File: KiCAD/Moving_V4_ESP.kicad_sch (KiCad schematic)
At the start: 88 parts, among them J1 Vin_1, J10 Conn_01x03_Pin, J11 Conn_01x03_Pin, J12 Conn_01x03_Pin, J13 Conn_01x03_Pin, J3 Power_SW, J4 USB_B_Micro, J5 MOTOR_R, J6 Motor_L, J7 Conn_01x04_Pin, J8 Conn_01x04_Pin, J9 Vin_XT, Q1 U4_ALT2, Q2 U4_ALT2, Q3 U4_ALT2, SW1 SW_Reset, U1 CH340X, U10 TXB0104RUT, U2 UZ1085L-33-TN3-R, U3 ESP32-WROOM-32, U4 ITR8307-S17-TR8, U5 ITR8307-S17-TR8, U6 ITR8307-S17-TR8, U7 CP3119MDTR, U8 CP2119LDTR, U9 SE8650K2B-HF

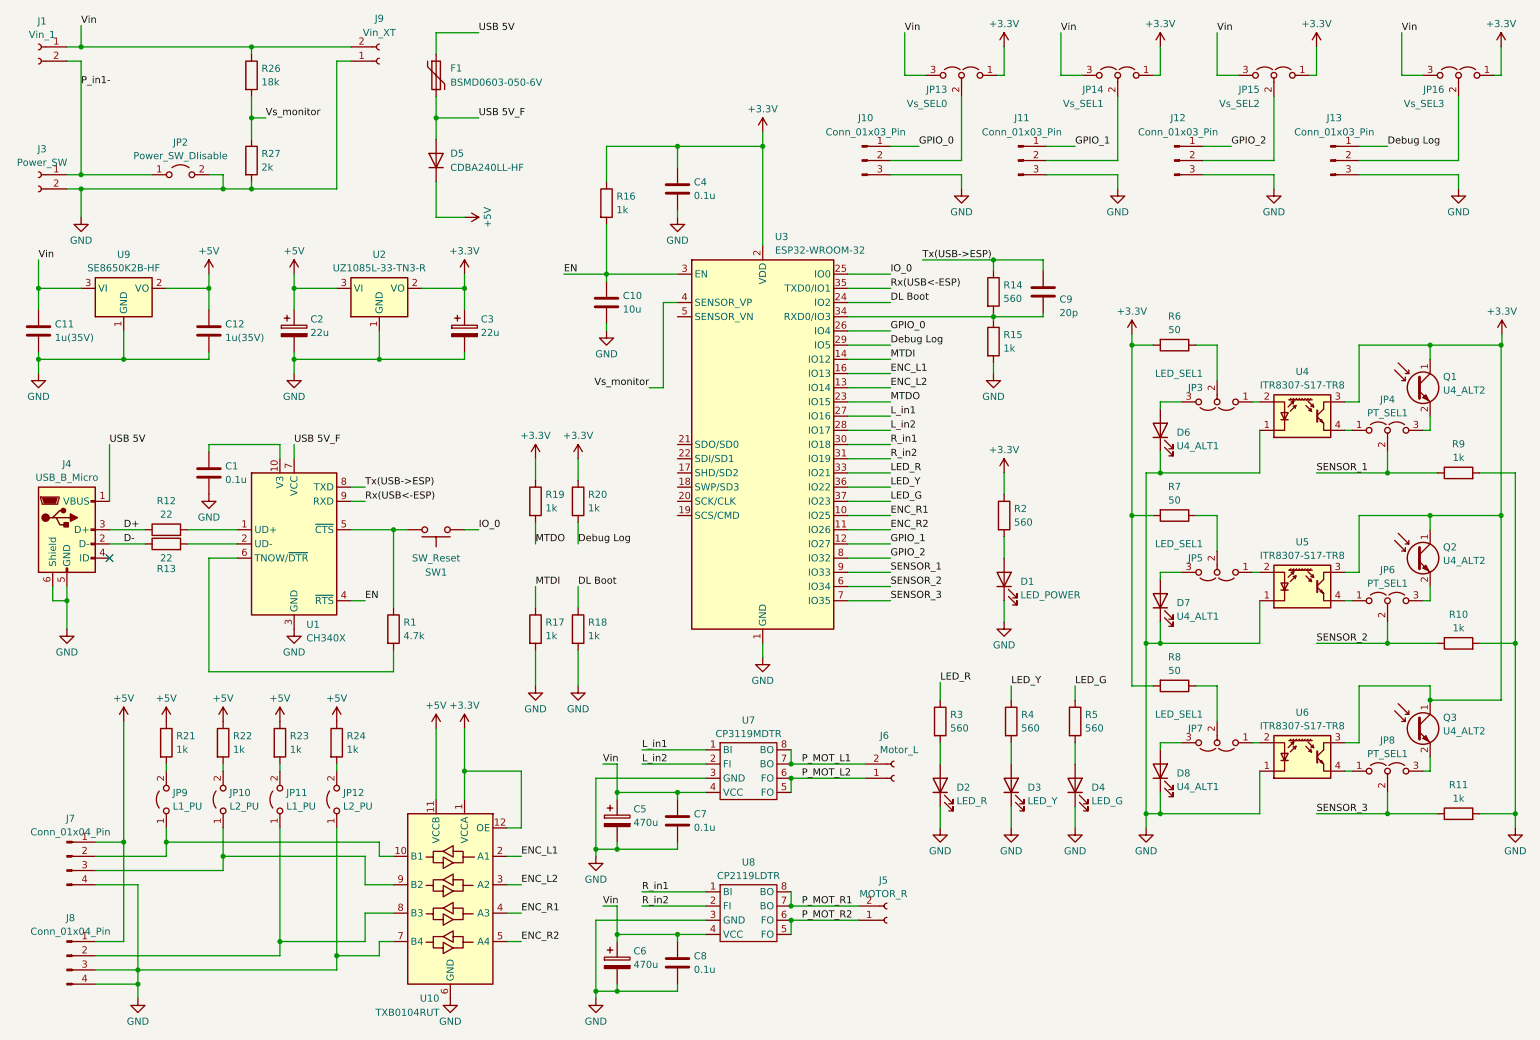
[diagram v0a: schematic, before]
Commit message: アノテーションを再実行
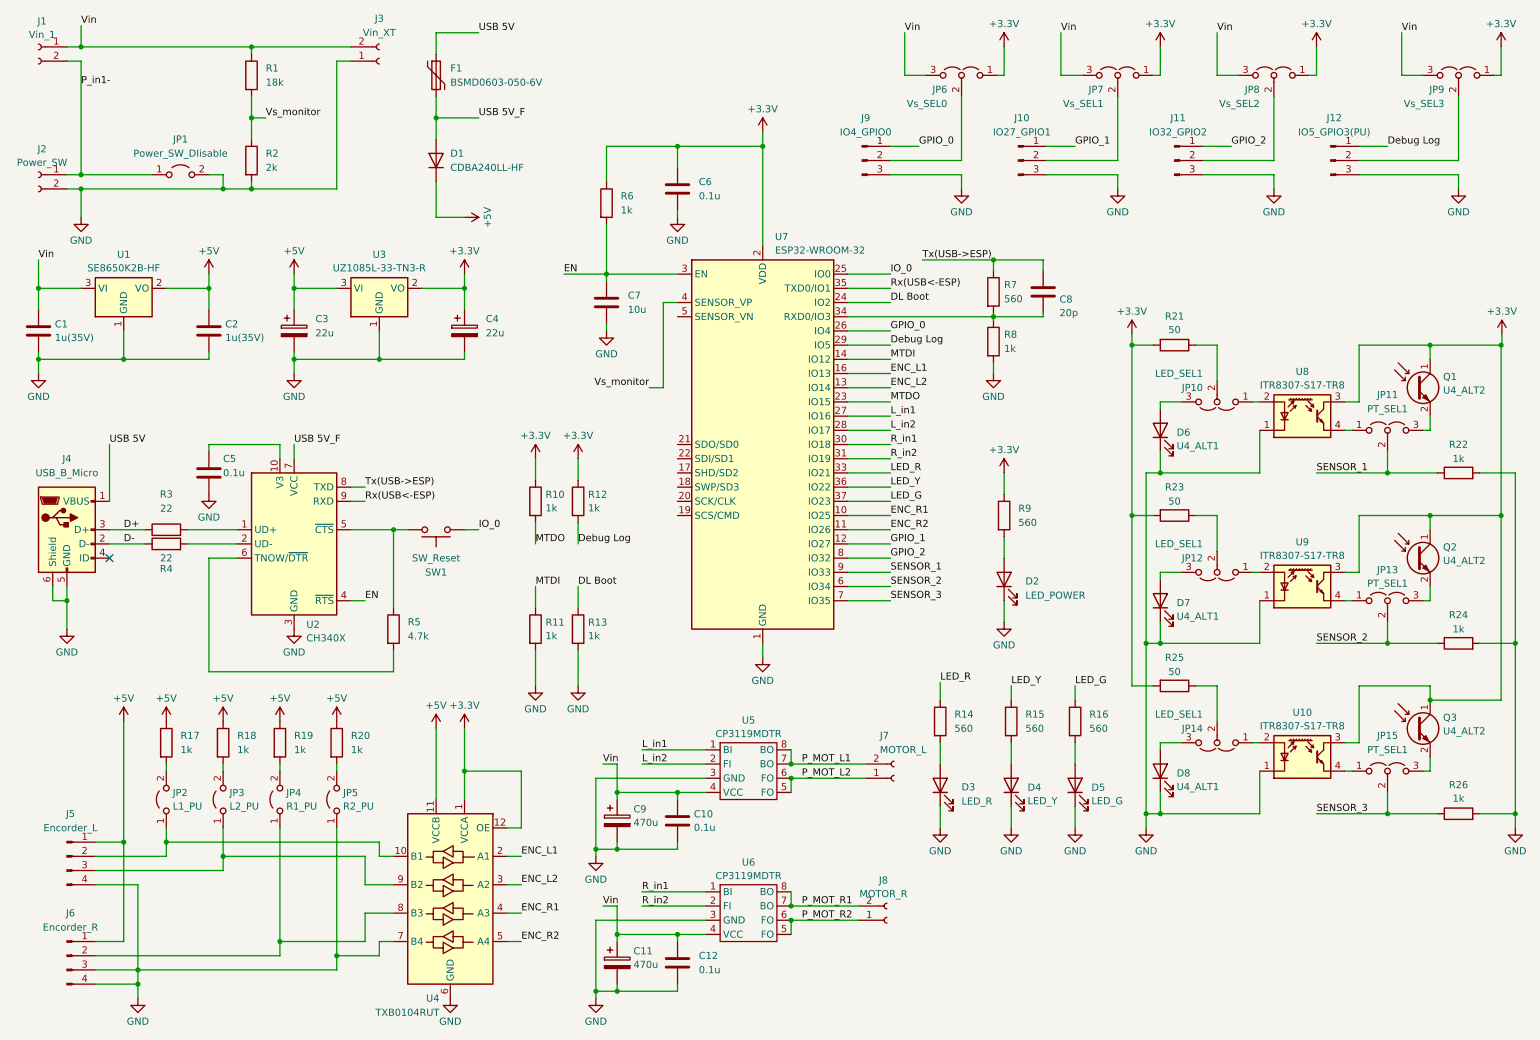
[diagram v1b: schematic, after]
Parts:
- J10: renamed from J11; value Conn_01x03_Pin -> IO27_GPIO1
- J11: renamed from J12; value Conn_01x03_Pin -> IO32_GPIO2
- J12: renamed from J13; value Conn_01x03_Pin -> IO5_GPIO3(PU)
- J5: renamed from J7; value Conn_01x04_Pin -> Encorder_L
- J6: renamed from J8; value Conn_01x04_Pin -> Encorder_R
- J7: renamed from J6; value Motor_L -> MOTOR_L
- J9: renamed from J10; value Conn_01x03_Pin -> IO4_GPIO0
- JP4: renamed from JP11; value L1_PU -> R1_PU
- JP5: renamed from JP12; value L2_PU -> R2_PU
- U6: renamed from U8; value CP2119LDTR -> CP3119MDTR
- renumbered C11 to C1, C7 to C10, C6 to C11, C8 to C12, C12 to C2, C2 to C3, C3 to C4, C1 to C5, C4 to C6, C10 to C7, C9 to C8, C5 to C9, D5 to D1, D1 to D2, D2 to D3, D3 to D4, D4 to D5, J3 to J2, J9 to J3, J5 to J8, JP2 to JP1, JP3 to JP10, JP4 to JP11, JP5 to JP12, JP6 to JP13, JP7 to JP14, JP8 to JP15, JP9 to JP2, JP10 to JP3, JP13 to JP6, JP14 to JP7, JP15 to JP8, JP16 to JP9, R26 to R1, R19 to R10, R17 to R11, R20 to R12, R18 to R13, R3 to R14, R4 to R15, R5 to R16, R21 to R17, R22 to R18, R23 to R19, R27 to R2, R24 to R20, R6 to R21, R9 to R22, R7 to R23, R10 to R24, R8 to R25, R11 to R26, R12 to R3, R13 to R4, R1 to R5, R16 to R6, R14 to R7, R15 to R8, R2 to R9, U9 to U1, U6 to U10, U1 to U2, U2 to U3, U10 to U4, U7 to U5, U3 to U7, U4 to U8, U5 to U9
